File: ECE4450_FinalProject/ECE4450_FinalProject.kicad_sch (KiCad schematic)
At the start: 19 parts, among them J1 PWR, J2 IN, J3 OUT, P1 Front_panel, Q1 BS250, U1 MAX1044, U2 SSM2164PZ, U3 TL072

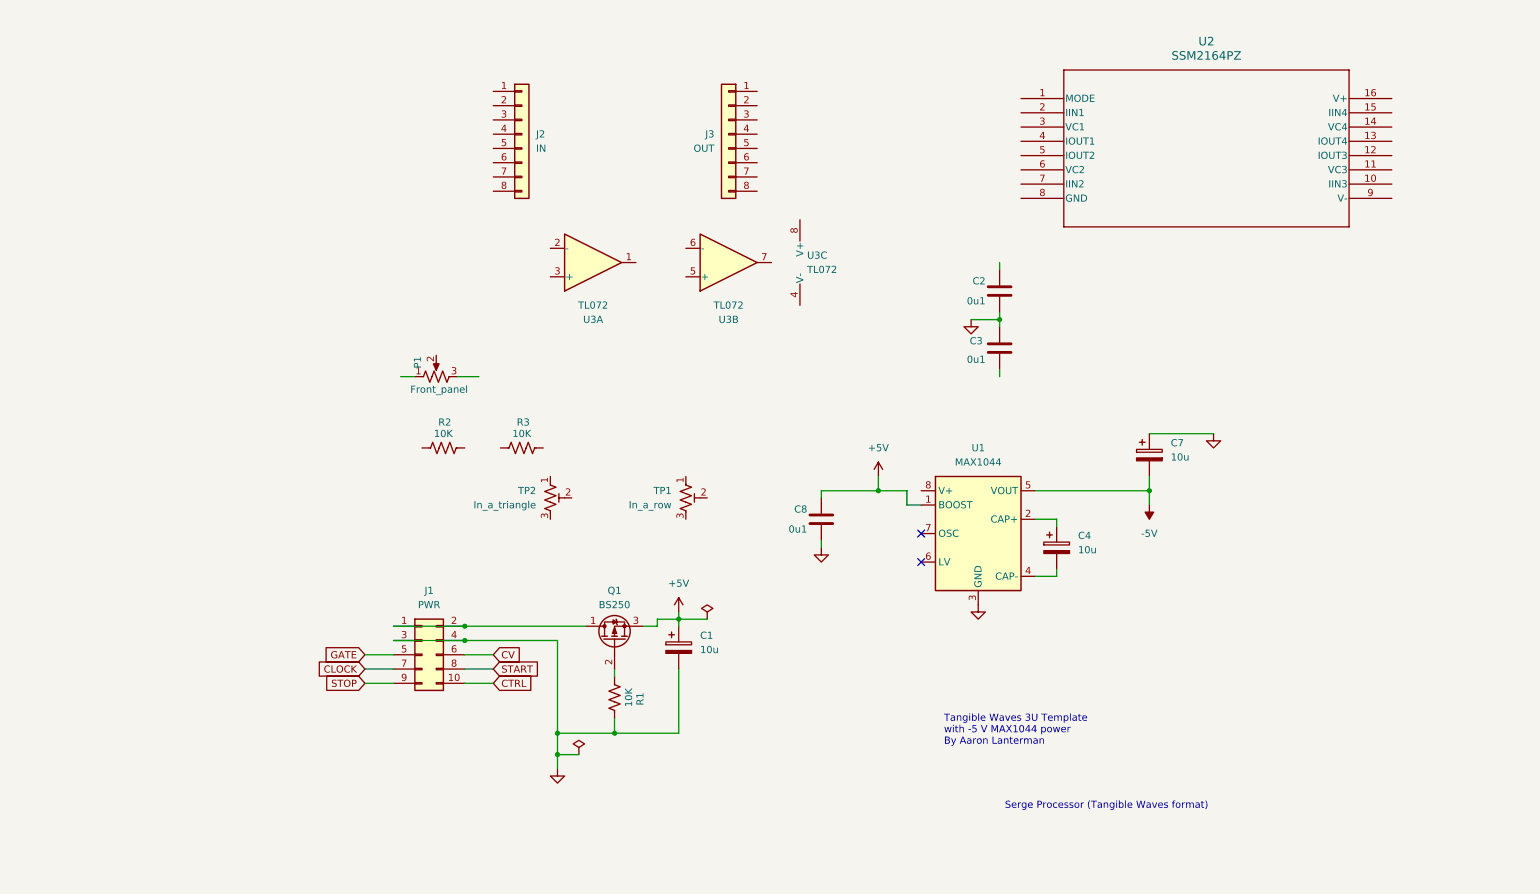
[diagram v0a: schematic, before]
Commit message: Add files via upload
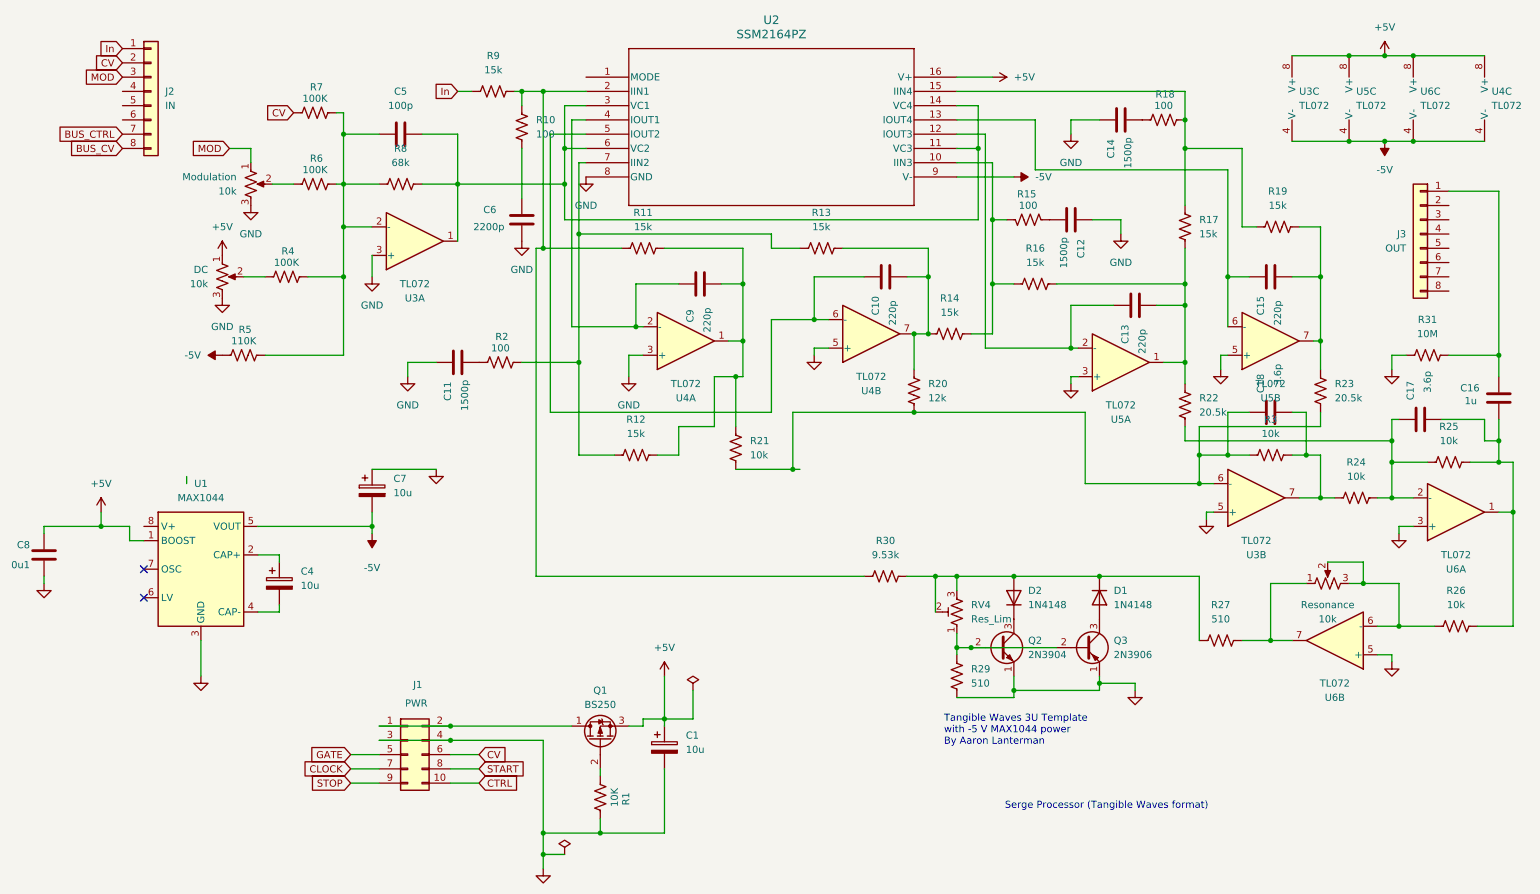
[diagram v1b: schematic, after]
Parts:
- removed C2, C3: 0u1, Aaron_Library:C_Axial_Aaron, symbol Device:C
- removed P1: Front_panel, Aaron_Library:Potentiometer_TW_Frontpanel, symbol Device:R_Potentiometer_US
- removed TP1: In_a_row, Potentiometer_THT:Potentiometer_Bourns_3296W_Vertical, symbol Device:R_Potentiometer_Trim_US
- removed TP2: In_a_triangle, Aaron_Library:Potentiometer_Square_Trimpot_Aaron, symbol Device:R_Potentiometer_Trim_US
- added C10, C13, C15, C9: 220p, symbol Device:C
- added C11, C12, C14: 1500p, symbol Device:C
- added C16: 1u, symbol Device:C
- added C17, C18: 3.6p, symbol Device:C
- added C5: 100p, symbol Device:C
- added C6: 2200p, symbol Device:C
- added D1, D2: 1N4148, Diode_THT:D_DO-35_SOD27_P7.62mm_Horizontal, symbol Diode:1N4148
- added DC, Modulation, Resonance: 10k, symbol Device:R_Potentiometer_US
- added Q2: 2N3904, Package_TO_SOT_THT:TO-92_Inline, symbol Transistor_BJT:2N3904
- added Q3: 2N3906, Package_TO_SOT_THT:TO-92_Inline, symbol Transistor_BJT:2N3906
- added R10: 100, symbol Device:R_US
- added R11, R12, R13, R14, R16, R17, R19, R9: 15k, symbol Device:R_US
- added R15, R18: 100, Aaron_Library:R_Axial_Aaron, symbol Device:R_US
- added R20: 12k, symbol Device:R_US
- added R21, R24, R25, R26: 10k, symbol Device:R_US
- added R22, R23: 20.5k, symbol Device:R_US
- added R27, R29: 510, symbol Device:R_US
- added R30: 9.53k, symbol Device:R_US
- added R31: 10M, symbol Device:R_US
- added R4, R6, R7: 100K, Aaron_Library:R_Axial_Aaron, symbol Device:R_US
- added R5: 110K, Aaron_Library:R_Axial_Aaron, symbol Device:R_US
- added R8: 68k, symbol Device:R_US
- added RV4: Res_Lim, symbol Device:R_Potentiometer_Trim_US
- added U4, U5, U6: TL072, symbol Amplifier_Operational:TL072
- R2: value 10K -> 100
- R3: value 10K -> 10k; footprint Aaron_Library:R_Axial_Aaron -> (none)
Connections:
- net +5V: now also U2.16 (V+), U3.8 (V+), DC.1, U4.8 (V+), U5.8 (V+), U6.8 (V+)
- net -5V: now also U2.9 (V-), U3.4 (V-), R5.2, U4.4 (V-), U5.4 (V-), U6.4 (V-)
- net CV: now also J2.2 (Pin_2), R7.2
- net GND: now also U2.8 (GND), U3.3 (+), U3.5 (+), C11.2, C12.2, C14.2, C6.1, DC.3, Modulation.3, Q2.1 (E), Q3.1 (E), R29.1, R31.1, U4.3 (+), U4.5 (+), U5.3 (+), U5.5 (+), U6.3 (+), U6.5 (+)
- net at U3.1: now also U2.11 (VC3), U2.14 (VC4), U2.3 (VC1), U2.6 (VC2), C5.2, R8.2
- net at U3.2 (-): now also C5.1, R4.1, R5.1, R6.1, R7.1, R8.1
- net at R2.1: now also U2.7 (IIN2), R12.1, R13.1
- net at R2.2: now also C11.1
- net at J3.1 (Pin_1): now also C16.2, R31.2
- net at U3.6 (-): now also R3.1, C18.2, R20.2, R21.2, R23.2
- net at U3.7: now also R3.2, C18.1, R24.1
- net at U2.10 (IIN3): now also R14.2, R15.1, R16.1
- net at U2.12 (IOUT3): now also C13.2, U5.2 (-)
- net at U2.13 (IOUT4): now also C15.2, U5.6 (-)
- net at U2.15 (IIN4): now also R17.2, R18.1, R19.2
- net at U2.2 (IIN1): now also R10.2, R11.1, R30.1, R9.2
- net at U2.4 (IOUT1): now also C9.2, U4.2 (-)
- net at U2.5 (IOUT2): now also C10.2, U4.6 (-)
- net In: now reaches J2.1 (Pin_1)
- net In: now also R9.1
- net MOD: now reaches J2.3 (Pin_3)
- net MOD: now also Modulation.1
- net BUS_CTRL: now reaches J2.7 (Pin_7)
- net BUS_CV: now reaches J2.8 (Pin_8)
- new net: Q2.2 (B), Q3.2 (B), R29.2, RV4.1
- new net: D2.1 (K), Q2.3 (C)
- new net: C14.1, R18.2
- new net: C13.1, R16.2, R17.1, R22.1, U5.1
- new net: R27.2, Resonance.1, U6.7
- new net: R26.1, Resonance.2, Resonance.3, U6.6 (-)
- new net: C10.1, R13.2, R14.1, R20.1, U4.7
- new net: C15.1, R19.1, R23.1, U5.7
- new net: C9.1, R11.2, R12.2, R21.1, U4.1
- new net: C6.2, R10.1
- new net: D1.2 (A), Q3.3 (C)
- new net: D1.1 (K), D2.2 (A), R27.1, R30.2, RV4.2, RV4.3
- new net: Modulation.2, R6.2
- new net: C17.2, R22.2, R24.2, R25.1, U6.2 (-)
- new net: C16.1, C17.1, R25.2, R26.2, U6.1
- new net: DC.2, R4.2
- new net: C12.1, R15.2
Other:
- moved on the sheet: C1, C4, C7, C8, J1, J2, J3, Q1, R1, R2, U1, U2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
